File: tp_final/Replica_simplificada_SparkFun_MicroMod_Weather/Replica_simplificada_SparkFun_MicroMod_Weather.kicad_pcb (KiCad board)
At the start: 2 copper layers, 38.7 x 40 mm, 32 parts, among them J1 USB_C_Receptacle_USB2.0, J2 Conn_01x05, J3 Conn_01x02, J4 Conn_01x03, U1 BME280, U2 AP7361C-33F, U3 AS3935

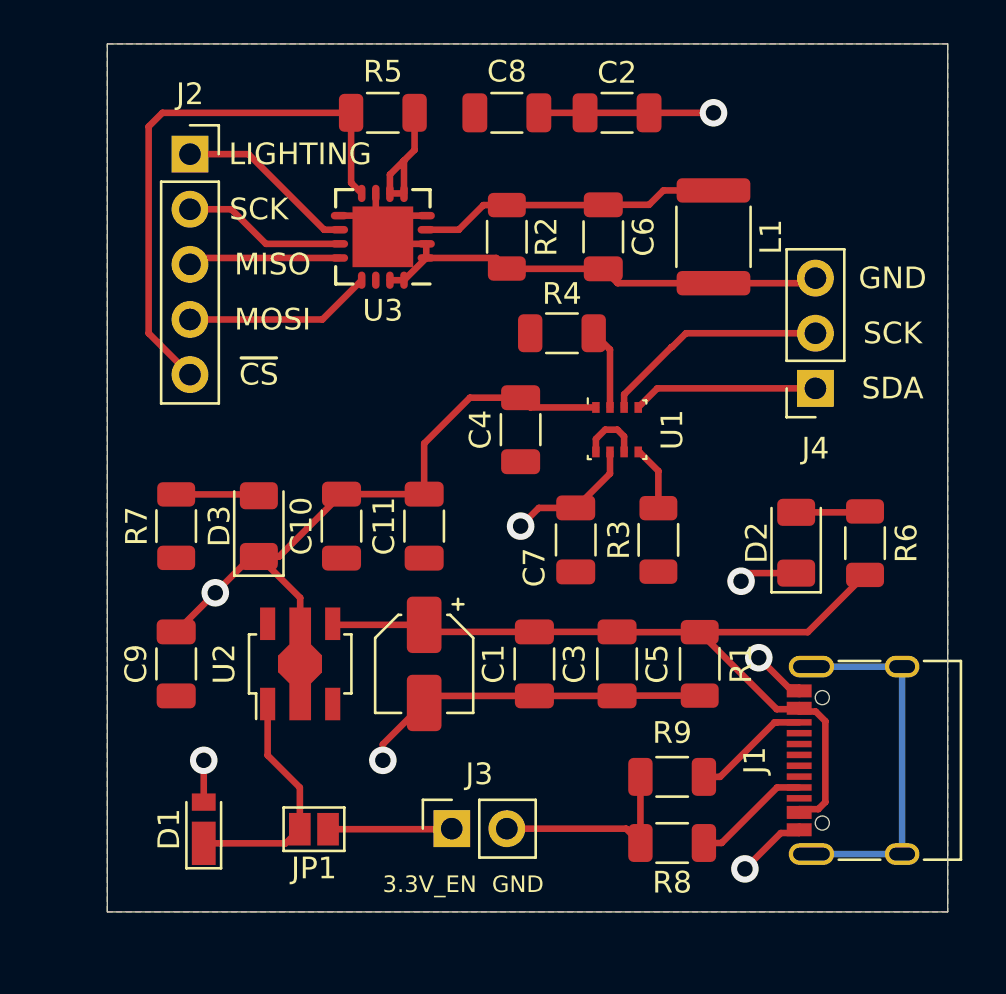
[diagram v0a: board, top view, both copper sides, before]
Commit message: Primeras correciones
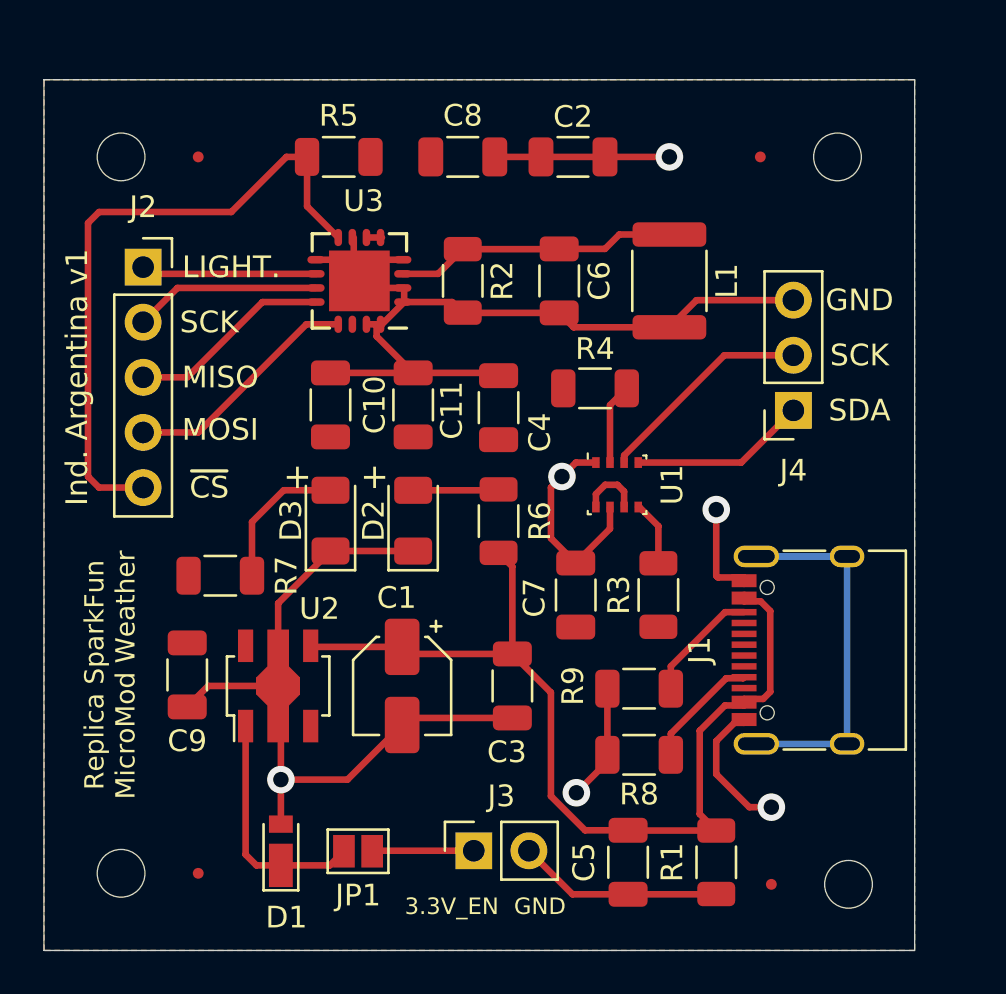
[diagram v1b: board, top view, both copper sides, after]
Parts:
- added REF**: Fiducial_0.5mm_Mask1.5mm, Fiducial:Fiducial_0.5mm_Mask1.5mm, F.Cu at (156.5, 83.3)
- added REF**: Fiducial_0.5mm_Mask1.5mm, Fiducial:Fiducial_0.5mm_Mask1.5mm, F.Cu at (130.6, 83.3)
- added REF**: Fiducial_0.5mm_Mask1.5mm, Fiducial:Fiducial_0.5mm_Mask1.5mm, F.Cu at (130.6, 116.3)
- added REF**: Fiducial_0.5mm_Mask1.5mm, Fiducial:Fiducial_0.5mm_Mask1.5mm, F.Cu at (157.0, 116.8)
- added REF**: MountingHole_2.2mm_M2_ISO7380, MountingHole:MountingHole_2.2mm_M2_ISO7380, F.Cu at (160.5, 116.8)
- added REF**: MountingHole_2.2mm_M2_ISO7380, MountingHole:MountingHole_2.2mm_M2_ISO7380, F.Cu at (127.0, 116.3)
- added REF**: MountingHole_2.2mm_M2_ISO7380, MountingHole:MountingHole_2.2mm_M2_ISO7380, F.Cu at (127.0, 83.3)
- added REF**: MountingHole_2.2mm_M2_ISO7380, MountingHole:MountingHole_2.2mm_M2_ISO7380, F.Cu at (160.0, 83.3)
- moved D2 17.7 mm to (140.5, 100.1)
- moved R6 16.9 mm to (144.4, 100.1)
- moved R1 9.18 mm to (154.4, 115.8)
- moved C5 9.16 mm to (150.4, 115.8)
- moved J1 5.68 mm to (159.4, 106.0)
- moved J2 5.64 mm to (128.0, 88.4)
- moved C10 5.61 mm to (136.7, 94.7)
- moved C11 5.61 mm to (140.5, 94.7)
- moved R8 4.34 mm to (150.9, 110.9)
- moved R9 4.34 mm to (150.9, 107.8)
- moved D1 3.70 mm to (134.4, 115.3)
- moved D3 3.31 mm to (136.7, 100.1)
- moved R7 3.06 mm to (131.6, 102.6), turned to 0 degrees
- moved R4 2.96 mm to (148.8, 94.0)
- moved C2 2.87 mm to (147.8, 83.3)
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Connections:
- J4 pad 1: I2C_SDA -> I2C_SCK
- J4 pad 2: I2C_SCK -> I2C_SDA
- U1 pad 3: I2C_SCK -> I2C_SDA
- U1 pad 4: I2C_SDA -> I2C_SCK
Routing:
- net GND: track 112.7 -> 119.8 mm, vias 8 -> 6
- net +3V3: track 9.25 -> 3.57 mm
- net +5V: track 38.9 -> 43.7 mm
- net /SPI_~CS~: track 25.7 -> 30.1 mm
- net Net-(D3-Pad2): track 3.84 -> 6.70 mm
- net I2C_SCK: track 10.6 -> 8.15 mm
- net /SPI_MISO: track 7.01 -> 9.41 mm
- net /SPI_MOSI: track 8.66 -> 11.1 mm
- net I2C_SDA: track 8.53 -> 10.0 mm
- net /SPI_SCK: track 7.55 -> 8.62 mm
- net 3.3V_EN: track 5.71 -> 4.69 mm
- net Net-(C6-Pad1): track 14.0 -> 13.0 mm
- net Net-(D2-Pad2): track 3.19 -> 3.95 mm
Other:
- board size 38.7 x 40 mm -> 40.1 x 40.1 mm
- board text added: "+"
- board text added: "Ind. Argentina v1"
- board text added: "LIGHT."
- board text added: "Margen: 6 mils Grilla: 20 mils"
- board text added: "Minimo ancho de pista: 5 mils Minimo diamtero via: 1.1 mm Minimo taladro: 0.5 mm"
- board text added: "Replica SparkFun MicroMod Weather"
- board text added: "Valores tomados en base a fabricante: Mayer PCB"
- board text removed: "LIGHTING"
